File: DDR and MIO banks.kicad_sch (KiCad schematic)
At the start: 42 parts, among them J4 Conn_01x04_Pin, J5 Conn_01x02_Pin, J8 Conn_01x02_Pin, U1 XC7Z020-1CLG400I__, U23 NC7WZ07P6X, Y2 SG-8018CE_50.0000M-TJHPA

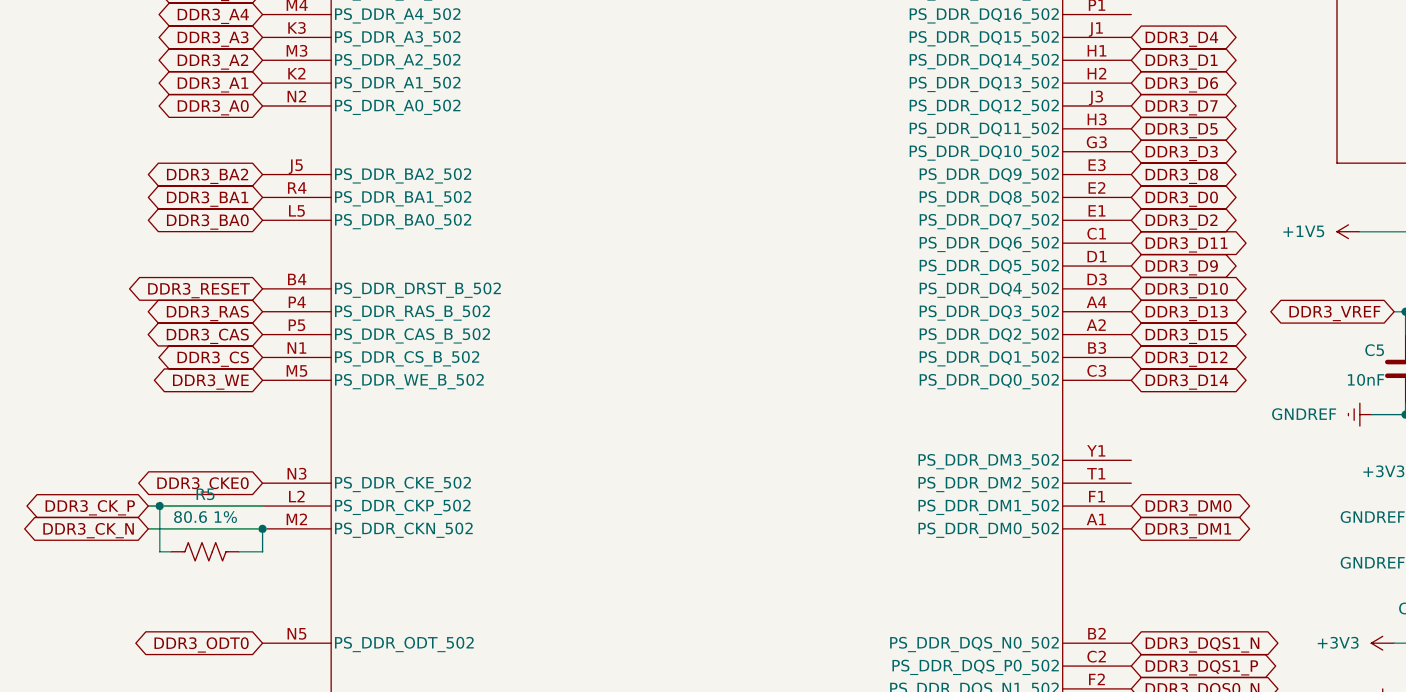
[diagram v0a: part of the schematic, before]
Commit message: update
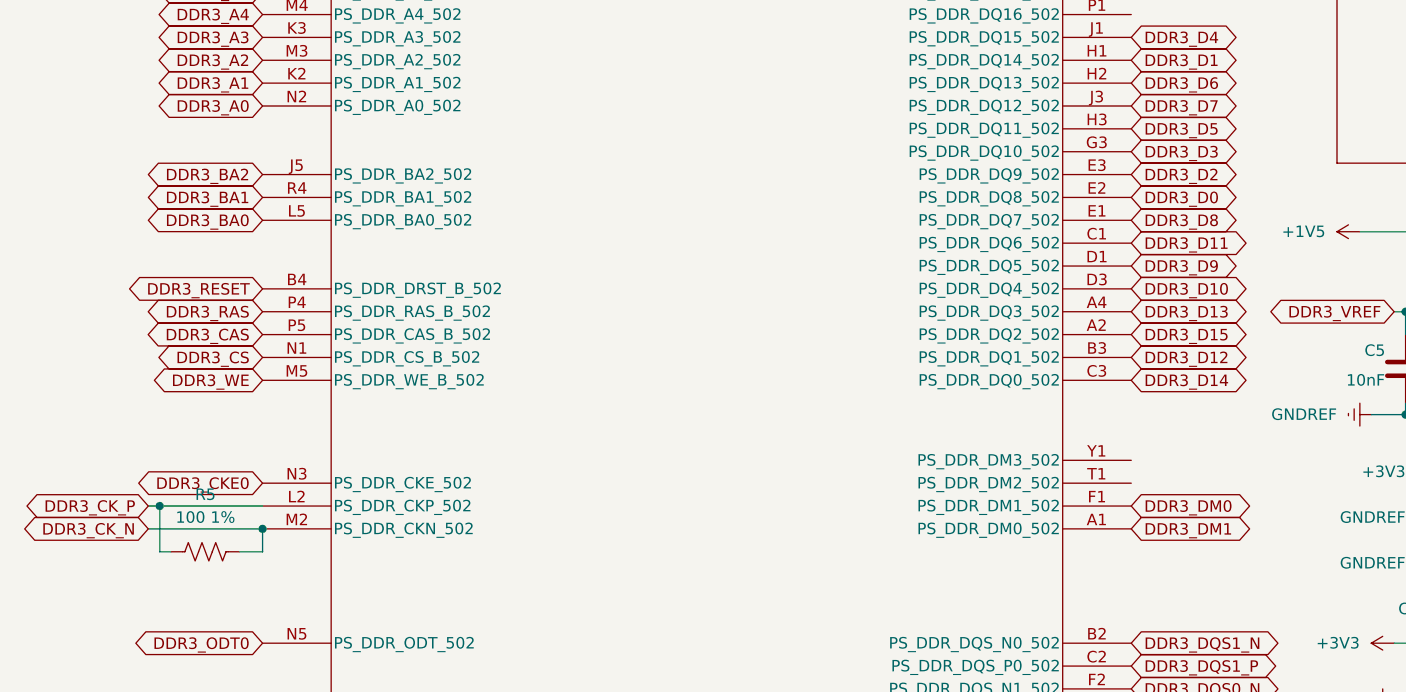
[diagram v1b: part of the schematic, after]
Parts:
- C8: footprint footprints:C_0402 -> footprints:C_0201_0603Metric
- R5: value 80.6 1% -> 100 1%
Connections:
- net DDR3_D2: now also U1.E3 (PS_DDR_DQ9_502); no longer U1.E1 (PS_DDR_DQ7_502)
- net DDR3_D8: now also U1.E1 (PS_DDR_DQ7_502); no longer U1.E3 (PS_DDR_DQ9_502)
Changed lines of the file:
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@@
 		)
 	)
-	(global_label "DDR3_D2"
+	(global_label "DDR3_D8"
 		(shape bidirectional)
 		(at 135.89 91.44 0)
@@
 		)
 	)
-	(global_label "DDR3_D8"
+	(global_label "DDR3_D2"
 		(shape bidirectional)
 		(at 135.89 86.36 0)
@@
 			)
 		)
-		(property "Value" "80.6 1%"
+		(property "Value" "100 1%"
 			(at 33.02 124.46 90)
 			(effects
@@
 			)
 		)
-		(property "Footprint" "footprints:C_0402"
+		(property "Footprint" "footprints:C_0201_0603Metric"
 			(at 200.3552 110.49 0)
 			(effects

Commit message: update
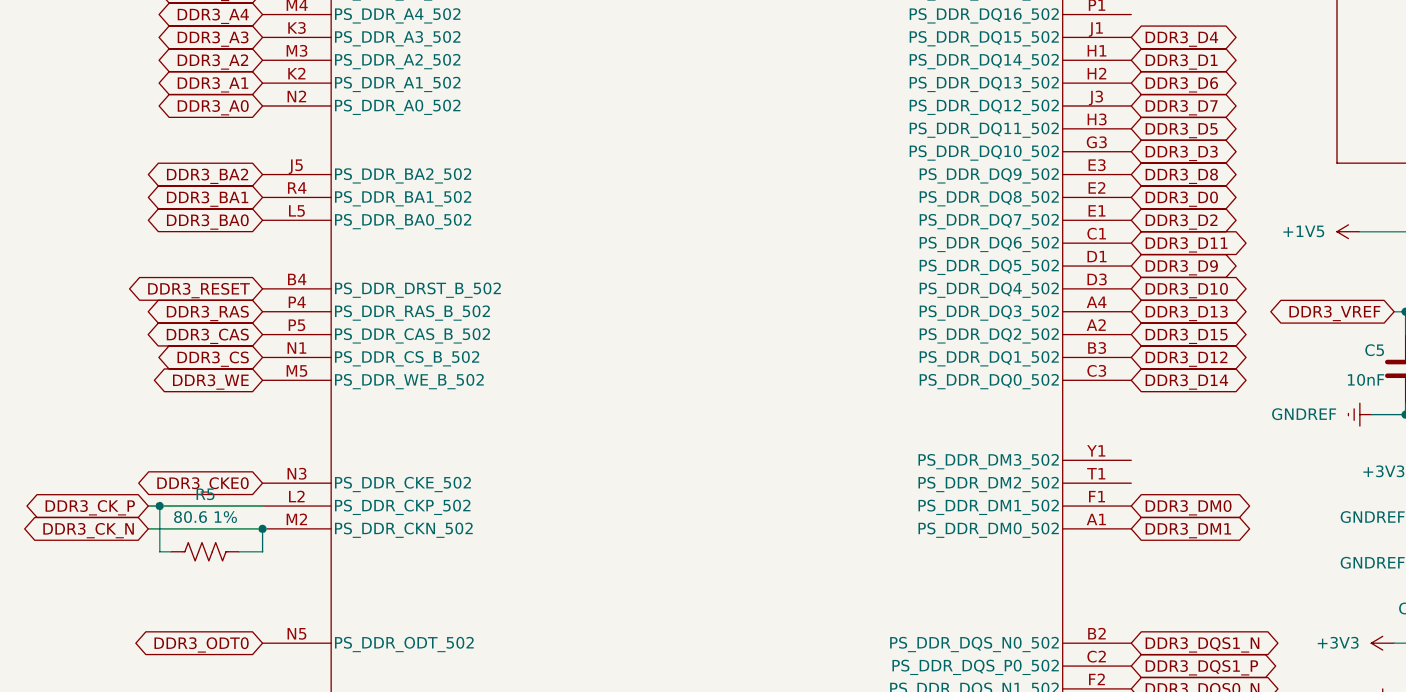
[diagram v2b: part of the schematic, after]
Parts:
- C8: footprint footprints:C_0201_0603Metric -> footprints:C_0402
- R5: value 100 1% -> 80.6 1%
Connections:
- net DDR3_D2: now also U1.E1 (PS_DDR_DQ7_502); no longer U1.E3 (PS_DDR_DQ9_502)
- net DDR3_D8: now also U1.E3 (PS_DDR_DQ9_502); no longer U1.E1 (PS_DDR_DQ7_502)
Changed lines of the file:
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@@
 		)
 	)
-	(global_label "DDR3_D8"
+	(global_label "DDR3_D2"
 		(shape bidirectional)
 		(at 135.89 91.44 0)
@@
 		)
 	)
-	(global_label "DDR3_D2"
+	(global_label "DDR3_D8"
 		(shape bidirectional)
 		(at 135.89 86.36 0)
@@
 			)
 		)
-		(property "Value" "100 1%"
+		(property "Value" "80.6 1%"
 			(at 33.02 124.46 90)
 			(effects
@@
 			)
 		)
-		(property "Footprint" "footprints:C_0201_0603Metric"
+		(property "Footprint" "footprints:C_0402"
 			(at 200.3552 110.49 0)
 			(effects

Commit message: Layout update
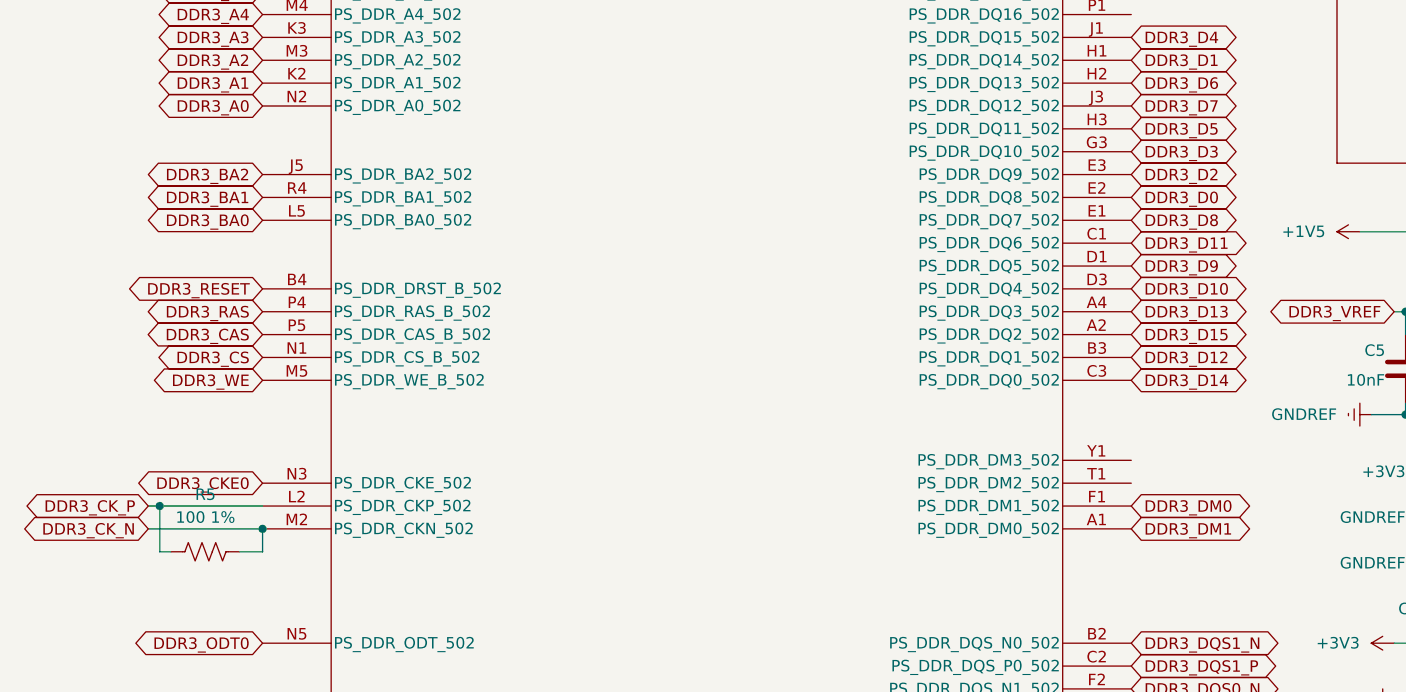
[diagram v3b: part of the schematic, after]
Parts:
- C8: footprint footprints:C_0402 -> footprints:C_0201_0603Metric
- R5: value 80.6 1% -> 100 1%
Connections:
- net DDR3_D2: now also U1.E3 (PS_DDR_DQ9_502); no longer U1.E1 (PS_DDR_DQ7_502)
- net DDR3_D8: now also U1.E1 (PS_DDR_DQ7_502); no longer U1.E3 (PS_DDR_DQ9_502)
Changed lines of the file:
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@@
 		)
 	)
-	(global_label "DDR3_D2"
+	(global_label "DDR3_D8"
 		(shape bidirectional)
 		(at 135.89 91.44 0)
@@
 		)
 	)
-	(global_label "DDR3_D8"
+	(global_label "DDR3_D2"
 		(shape bidirectional)
 		(at 135.89 86.36 0)
@@
 			)
 		)
-		(property "Value" "80.6 1%"
+		(property "Value" "100 1%"
 			(at 33.02 124.46 90)
 			(effects
@@
 			)
 		)
-		(property "Footprint" "footprints:C_0402"
+		(property "Footprint" "footprints:C_0201_0603Metric"
 			(at 200.3552 110.49 0)
 			(effects
